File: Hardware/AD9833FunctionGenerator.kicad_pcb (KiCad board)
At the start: 2 copper layers, 161.3 x 114.3 mm, 52 parts, among them U1 LM7805_TO220

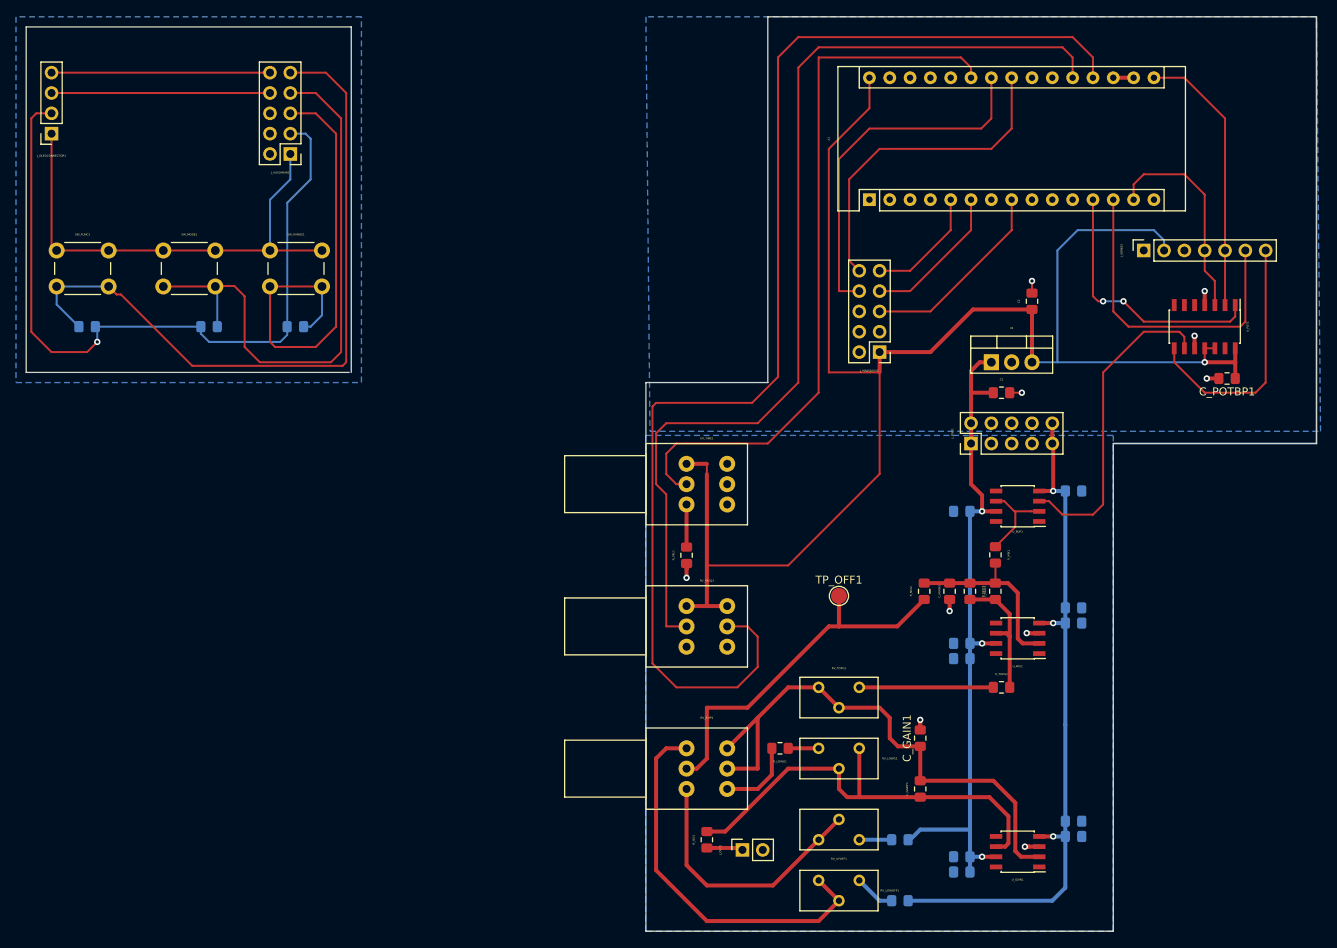
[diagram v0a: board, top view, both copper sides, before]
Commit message: board rev b
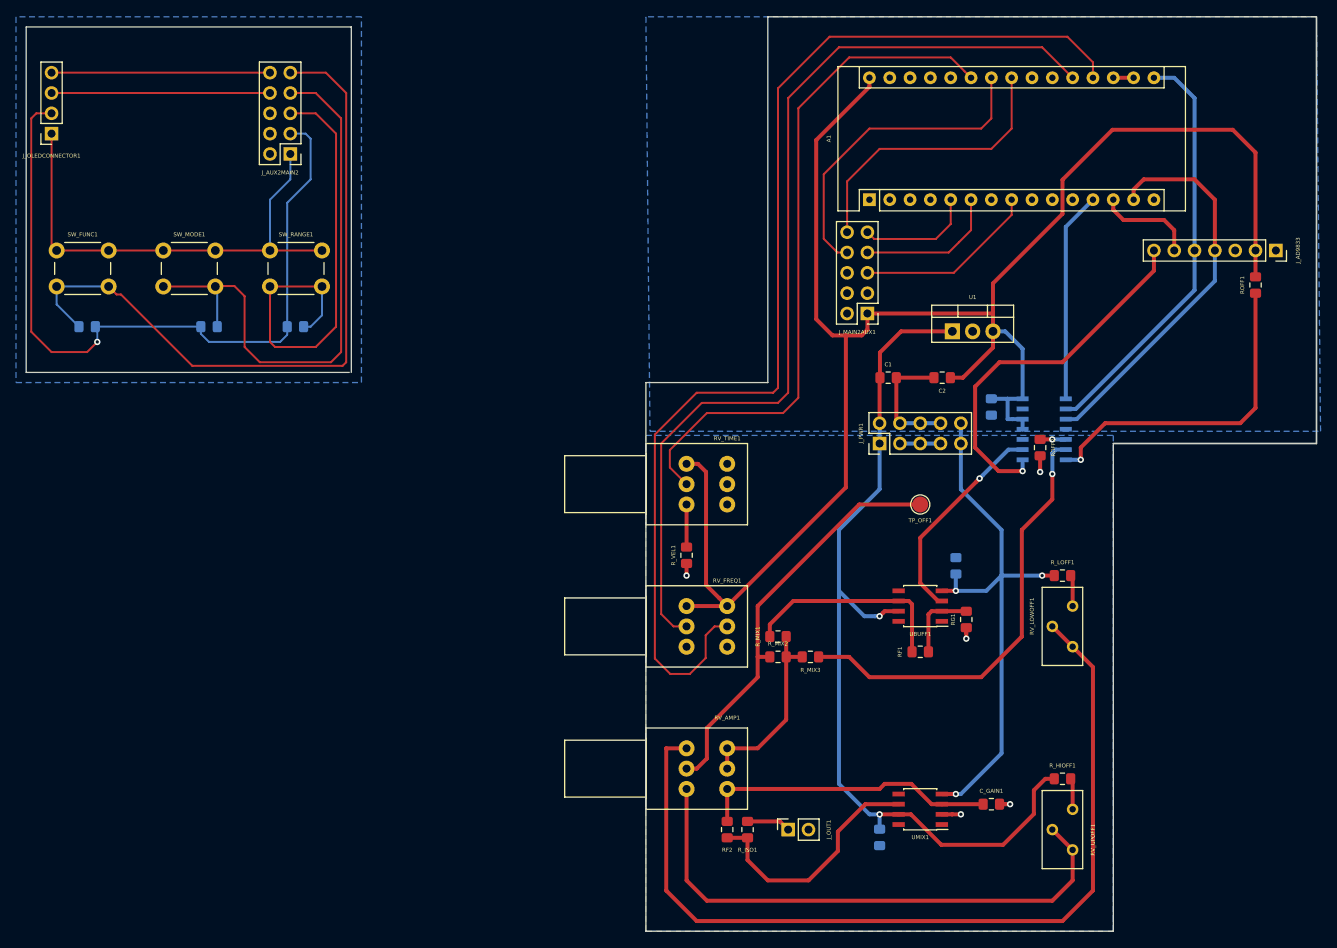
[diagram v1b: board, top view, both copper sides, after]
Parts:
- removed C_BUFBP1, C_BUFBP2: 100nF, Capacitor_SMD:C_0805_2012Metric_Pad1.15x1.40mm_HandSolder
- removed C_GAINBP1, C_GAINBP4, C_MIXBP1: 2.2uF TANT., Capacitor_SMD:C_0805_2012Metric_Pad1.15x1.40mm_HandSolder
- removed C_GAINBP2, C_GAINBP3, C_MIXBP2, C_MIXBP3: 10nF, Capacitor_SMD:C_0805_2012Metric_Pad1.15x1.40mm_HandSolder
- removed C_GAINF1, C_MIXF1, C_MIXIN1: ?, Capacitor_SMD:C_0805_2012Metric_Pad1.15x1.40mm_HandSolder
- removed C_MIXBP4: 2.2pF TANT., Capacitor_SMD:C_0805_2012Metric_Pad1.15x1.40mm_HandSolder
- removed RV_LOWG1: 100R, Potentiometer_THT:Potentiometer_Bourns_3296Y_Vertical
- removed RV_TOPG1: 10K, Potentiometer_THT:Potentiometer_Bourns_3296Y_Vertical
- removed R_LOWG1: 120R, Resistor_SMD:R_0805_2012Metric_Pad1.15x1.40mm_HandSolder
- removed R_MIXF1: 10K, Resistor_SMD:R_0805_2012Metric_Pad1.15x1.40mm_HandSolder
- removed R_TOPG1: 330R, Resistor_SMD:R_0805_2012Metric_Pad1.15x1.40mm_HandSolder
- removed U_BUF1: TL071, Package_SO:SOIC-8_3.9x4.9mm_P1.27mm
- removed U_GAIN1, U_MIX1: LM7171, Package_SO:SOIC-8_3.9x4.9mm_P1.27mm
- added C_BUFFBP1: 100nF, Capacitor_SMD:C_0805_2012Metric_Pad1.15x1.40mm_HandSolder, B.Cu at (148.6, 138.1)
- added C_BUFFBP2: 100nF, Capacitor_SMD:C_0805_2012Metric_Pad1.15x1.40mm_HandSolder, B.Cu at (158.1, 104.2)
- added RF1: 1k, Resistor_SMD:R_0805_2012Metric_Pad1.15x1.40mm_HandSolder, F.Cu at (153.7, 114.9)
- added RF2: 8K2, Resistor_SMD:R_0805_2012Metric_Pad1.15x1.40mm_HandSolder, F.Cu at (129.5, 137.2)
- added RG1: 1k, Resistor_SMD:R_0805_2012Metric_Pad1.15x1.40mm_HandSolder, F.Cu at (159.4, 110.9)
- added ROFF1: 1K, Resistor_SMD:R_0805_2012Metric_Pad1.15x1.40mm_HandSolder, F.Cu at (195.6, 69.1)
- added ROFF2: 1K, Resistor_SMD:R_0805_2012Metric_Pad1.15x1.40mm_HandSolder, F.Cu at (168.7, 89.4)
- added R_MIX3: 1K, Resistor_SMD:R_0805_2012Metric_Pad1.15x1.40mm_HandSolder, F.Cu at (139.9, 115.6)
- added UBUFF1: LT1227, Package_SO:SOIC-8_3.9x4.9mm_P1.27mm, F.Cu at (153.7, 109.2)
- added UMIX1: LT1227, Package_SO:SOIC-8_3.9x4.9mm_P1.27mm, F.Cu at (153.7, 134.6)
- C_POTBP1, U_POT1: moved to B.Cu
- R_HIOFF1, R_LOFF1: value 220R -> 1K; moved to F.Cu
- R_MIX1, R_MIX2: value 10K -> 1K
- moved R_LOFF1 45.4 mm to (171.4, 105.4), turned to 0 degrees
- moved RV_LOWOFF1 39.6 mm to (172.7, 114.3), turned to 270 degrees
- moved RV_UPOFF1 31.8 mm to (172.7, 139.7), turned to 270 degrees
- moved C_POTBP1 29.7 mm to (162.6, 84.3), turned to 270 degrees
- moved R_MIX1 29.0 mm to (135.9, 113.0), turned to 0 degrees
- moved U_POT1 23.8 mm to (169.2, 87.1), turned to 180 degrees
- moved R_HIOFF1 21.7 mm to (171.4, 130.8), turned to 0 degrees
- moved R_MIX2 20.0 mm to (135.9, 115.6), turned to 0 degrees
- moved J_AD9833 16.5 mm to (198.1, 64.8), turned to 270 degrees
- moved TP_OFF1 15.3 mm to (153.7, 96.5), turned to 180 degrees
- moved C2 14.7 mm to (156.4, 80.7), turned to 180 degrees
- moved C1 14.3 mm to (149.7, 80.7)
- moved C_GAIN1 12.1 mm to (162.6, 134.0), turned to 0 degrees
- moved J_PWR1 11.4 mm to (148.6, 88.9)
- moved J_OUT1 6.25 mm to (137.2, 137.2)
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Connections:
- RV_AMP1 pad 4: Net-(RV_AMP1-Pad4) -> Net-(C_GAIN1-Pad1)
- RV_AMP1 pad 5: Net-(C_GAIN1-Pad1) -> Net-(RV_AMP1-Pad5)
- RV_AMP1 pad 6: Net-(C_GAIN1-Pad1) -> Net-(RV_AMP1-Pad5)
- RV_LOWOFF1 pad 1: Net-(RV_LOWOFF1-Pad1) -> Net-(RV_AMP1-Pad3)
- RV_LOWOFF1 pad 3: Net-(RV_AMP1-Pad3) -> Net-(RV_LOWOFF1-Pad3)
- R_LOFF1 pad 2: Net-(RV_LOWOFF1-Pad1) -> Net-(RV_LOWOFF1-Pad3)
- R_MIX1 pad 2: Net-(C_MIXF1-Pad2) -> Net-(RV_AMP1-Pad5)
- R_MIX2 pad 2: Net-(C_MIXF1-Pad2) -> Net-(RV_AMP1-Pad5)
- U_POT1 pad 10: /GND -> /AGND
- U_POT1 pad 5: (no net) -> Net-(ROFF2-Pad1)
- U_POT1 pad 6: (no net) -> /OFFSETADJUST
- U_POT1 pad 7: (no net) -> Net-(ROFF1-Pad1)
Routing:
- net Net-(RV_AMP1-Pad3): track 48.4 -> 111.9 mm
- net /OFFSETADJUST: track 0.00 -> 54.9 mm, vias 0 -> 1
- net Net-(ROFF1-Pad1): track 0.00 -> 41.6 mm, vias 0 -> 1
- net Net-(RV_AMP1-Pad1): track 33.0 -> 69.2 mm
- net Net-(C_GAIN1-Pad1): track 68.4 -> 37.4 mm
- net /DDS_CS: track 40.4 -> 12.5 mm
- net Net-(RF2-Pad1): track 56.1 -> 30.6 mm
- net /+12V: track 87.4 -> 112.3 mm, vias 3 -> 2
- net Net-(RV_AMP1-Pad5): track 0.00 -> 23.8 mm
- net Net-(C_MIXF1-Pad2): track 23.4 -> 0.00 mm
- net /MOSI: track 26.7 -> 49.0 mm
- net /-12V: track 88.0 -> 69.9 mm
- net /SCK: track 34.3 -> 51.9 mm
- net Net-(C_MIXF1-Pad1): track 16.8 -> 0.00 mm
- net Net-(RV_TOPG1-Pad1): track 16.8 -> 0.00 mm
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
